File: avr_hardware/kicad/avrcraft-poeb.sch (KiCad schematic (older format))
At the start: 61 parts, among them J1 AVRISP6, J2 AVRISP6, P1 ETHERNET, P4 GND, P5 PD34, P6 5V, P7 3V3, P8 PB0, Q1 SQ2361EES-T1-GE3CT-ND, T1 S553-5999-52, U1 ATMEGA328, U2 MCP1824v3.3, U3 ENC424J600, U4 A4447SLJTR, X1 XTAL4P, X2 25MHz

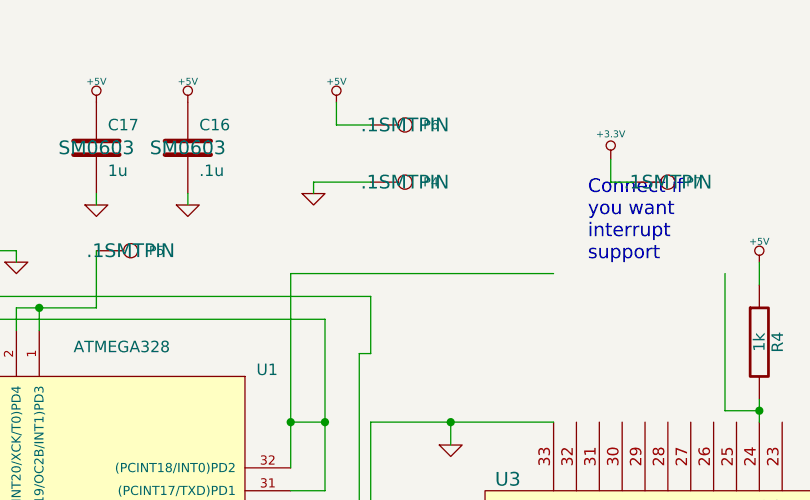
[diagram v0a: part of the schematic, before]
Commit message: update poc
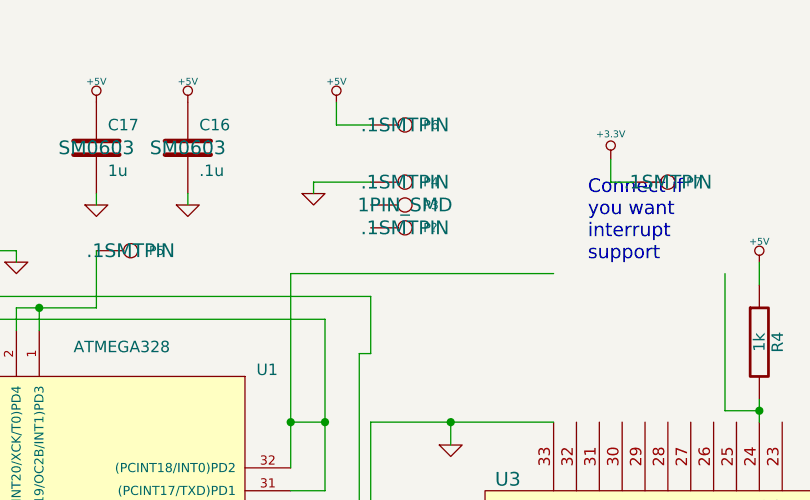
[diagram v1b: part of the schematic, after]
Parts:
- added P3: GND, 1PIN_SMD, symbol CONN_1
- added P?: GND, .1SMTPIN, symbol CONN_1
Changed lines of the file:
@@
-EESchema Schematic File Version 2  date Wed 27 Nov 2013 03:16:10 PM EST
+EESchema Schematic File Version 2  date Tue 04 Feb 2014 05:22:17 PM EST
 LIBS:power
 LIBS:device
@@
 Sheet 1 1
 Title ""
-Date "27 nov 2013"
+Date "4 feb 2014"
 Rev ""
 Comp ""
@@
 Connection ~ 1850 550
 $Comp
-L GND #PWR01
+L CONN_1 P?
+U 1 1 52F167B0
+P 5400 1450
+F 0 "P?" H 5480 1450 40  0000 L CNN
+F 1 "GND" H 5400 1505 30  0001 C CNN
+F 2 ".1SMTPIN" H 5400 1450 60  0000 C CNN
+	1    5400 1450
+	1    0    0    -1
+$EndComp
+$Comp
+L CONN_1 P3
+U 1 1 52F167AD
+P 5400 1350
+F 0 "P3" H 5480 1350 40  0000 L CNN
+F 1 "GND" H 5400 1405 30  0001 C CNN
+F 2 "1PIN_SMD" H 5400 1350 60  0000 C CNN
+	1    5400 1350
+	1    0    0    -1
+$EndComp
+$Comp
+L GND #PWR4
 U 1 1 52054D0F
 P 1950 1650
-F 0 "#PWR01" H 1950 1650 30  0001 C CNN
+F 0 "#PWR4" H 1950 1650 30  0001 C CNN
 F 1 "GND" H 1950 1580 30  0001 C CNN
 	1    1950 1650
@@
 $EndComp
 $Comp
-L +3.3V #PWR02
+L +3.3V #PWR3
 U 1 1 51D472BC
 P 1750 1900
-F 0 "#PWR02" H 1750 1860 30  0001 C CNN
+F 0 "#PWR3" H 1750 1860 30  0001 C CNN
 F 1 "+3.3V" H 1750 2010 30  0000 C CNN
 	1    1750 1900
@@
 $EndComp
 $Comp
-L GND #PWR03
+L GND #PWR31
 U 1 1 510EC704
 P 8000 2650
-F 0 "#PWR03" H 8000 2650 30  0001 C CNN
+F 0 "#PWR31" H 8000 2650 30  0001 C CNN
 F 1 "GND" H 8000 2580 30  0001 C CNN
 	1    8000 2650
@@
 Connect if \nyou want\ninterrupt\nsupport
 $Comp
-L +5V #PWR04
+L +5V #PWR24
 U 1 1 510EAED6
 P 6950 1600
-F 0 "#PWR04" H 6950 1690 20  0001 C CNN
+F 0 "#PWR24" H 6950 1690 20  0001 C CNN
 F 1 "+5V" H 6950 1690 30  0000 C CNN
 	1    6950 1600
@@
 $EndComp
 $Comp
-L +5V #PWR05
+L +5V #PWR11
 U 1 1 5109F491
 P 4050 900
-F 0 "#PWR05" H 4050 990 20  0001 C CNN
+F 0 "#PWR11" H 4050 990 20  0001 C CNN
 F 1 "+5V" H 4050 990 30  0000 C CNN
 	1    4050 900
@@
 $EndComp
 $Comp
-L GND #PWR06
+L GND #PWR12
 U 1 1 5109F490
 P 4050 1350
-F 0 "#PWR06" H 4050 1350 30  0001 C CNN
+F 0 "#PWR12" H 4050 1350 30  0001 C CNN
 F 1 "GND" H 4050 1280 30  0001 C CNN
 	1    4050 1350
@@
 NOTE: 5v Rail should be roughly 4.5V
 $Comp
-L GND #PWR07
+L GND #PWR14
 U 1 1 51031CF0
 P 4450 1350
-F 0 "#PWR07" H 4450 1350 30  0001 C CNN
+F 0 "#PWR14" H 4450 1350 30  0001 C CNN
 F 1 "GND" H 4450 1280 30  0001 C CNN
 	1    4450 1350
@@
 $EndComp
 $Comp
-L +5V #PWR08
+L +5V #PWR13
 U 1 1 51031CE7
 P 4450 900
-F 0 "#PWR08" H 4450 990 20  0001 C CNN
+F 0 "#PWR13" H 4450 990 20  0001 C CNN
 F 1 "+5V" H 4450 990 30  0000 C CNN
 	1    4450 900
@@
 $EndComp
 $Comp
-L +5V #PWR09
+L +5V #PWR16
 U 1 1 5102E4BB
 P 5100 900
-F 0 "#PWR09" H 5100 990 20  0001 C CNN
+F 0 "#PWR16" H 5100 990 20  0001 C CNN
 F 1 "+5V" H 5100 990 30  0000 C CNN
 	1    5100 900
@@
 $EndComp
 $Comp
-L +3.3V #PWR010
+L +3.3V #PWR22
 U 1 1 5102E4A4
 P 6300 1150
-F 0 "#PWR010" H 6300 1110 30  0001 C CNN
+F 0 "#PWR22" H 6300 1110 30  0001 C CNN
 F 1 "+3.3V" H 6300 1260 30  0000 C CNN
 	1    6300 1150
@@
 $EndComp
 $Comp
-L GND #PWR011
+L GND #PWR15
 U 1 1 5102E175
 P 5000 1300
-F 0 "#PWR011" H 5000 1300 30  0001 C CNN
+F 0 "#PWR15" H 5000 1300 30  0001 C CNN
 F 1 "GND" H 5000 1230 30  0001 C CNN
 	1    5000 1300
@@
 HighCOut
 $Comp
-L +5V #PWR012
+L +5V #PWR32
 U 1 1 5101B419
 P 8150 6850
-F 0 "#PWR012" H 8150 6940 20  0001 C CNN
+F 0 "#PWR32" H 8150 6940 20  0001 C CNN
 F 1 "+5V" H 8150 6940 30  0000 C CNN
 	1    8150 6850
@@
 $EndComp
 $Comp
-L GND #PWR013
+L GND #PWR21
 U 1 1 5101B3F2
 P 5700 7250
-F 0 "#PWR013" H 5700 7250 30  0001 C CNN
+F 0 "#PWR21" H 5700 7250 30  0001 C CNN
 F 1 "GND" H 5700 7180 30  0001 C CNN
 	1    5700 7250
@@
 POE+
 $Comp
-L GND #PWR014
+L GND #PWR34
 U 1 1 510061F7
 P 8750 6150
-F 0 "#PWR014" H 8750 6150 30  0001 C CNN
+F 0 "#PWR34" H 8750 6150 30  0001 C CNN
 F 1 "GND" H 8750 6080 30  0001 C CNN
 	1    8750 6150
@@
 $EndComp
 $Comp
-L GND #PWR015
+L GND #PWR35
 U 1 1 51005EDF
 P 10450 3050
-F 0 "#PWR015" H 10450 3050 30  0001 C CNN
+F 0 "#PWR35" H 10450 3050 30  0001 C CNN
 F 1 "GND" H 10450 2980 30  0001 C CNN
 	1    10450 3050
@@
 $EndComp
 $Comp
-L +3.3V #PWR016
+L +3.3V #PWR29
 U 1 1 50FE1DE9
 P 7950 5250
-F 0 "#PWR016" H 7950 5210 30  0001 C CNN
+F 0 "#PWR29" H 7950 5210 30  0001 C CNN
 F 1 "+3.3V" H 7950 5360 30  0000 C CNN
 	1    7950 5250
@@
 $EndComp
 $Comp
-L GND #PWR017
+L GND #PWR30
 U 1 1 50FE1DDF
 P 7950 5700
-F 0 "#PWR017" H 7950 5700 30  0001 C CNN
+F 0 "#PWR30" H 7950 5700 30  0001 C CNN
 F 1 "GND" H 7950 5630 30  0001 C CNN
 	1    7950 5700
@@
 $EndComp
 $Comp
-L GND #PWR018
+L GND #PWR33
 U 1 1 50FE1DDB
 P 8650 5000
-F 0 "#PWR018" H 8650 5000 30  0001 C CNN
+F 0 "#PWR33" H 8650 5000 30  0001 C CNN
 F 1 "GND" H 8650 4930 30  0001 C CNN
 	1    8650 5000
@@
 $EndComp
 $Comp
-L +3.3V #PWR019
+L +3.3V #PWR27
 U 1 1 50FDE179
 P 7750 2700
-F 0 "#PWR019" H 7750 2660 30  0001 C CNN
+F 0 "#PWR27" H 7750 2660 30  0001 C CNN
 F 1 "+3.3V" H 7750 2810 30  0000 C CNN
 	1    7750 2700
@@
 $EndComp
 $Comp
-L GND #PWR020
+L GND #PWR28
 U 1 1 50FDE152
 P 7800 4050
-F 0 "#PWR020" H 7800 4050 30  0001 C CNN
+F 0 "#PWR28" H 7800 4050 30  0001 C CNN
 F 1 "GND" H 7800 3980 30  0001 C CNN
 	1    7800 4050
@@
 $EndComp
 $Comp
-L GND #PWR021
+L GND #PWR26
 U 1 1 50FDE072
 P 7400 5150
-F 0 "#PWR021" H 7400 5150 30  0001 C CNN
+F 0 "#PWR26" H 7400 5150 30  0001 C CNN
 F 1 "GND" H 7400 5080 30  0001 C CNN
 	1    7400 5150
@@
 $EndComp
 $Comp
-L +5V #PWR022
+L +5V #PWR9
 U 1 1 50FDE020
 P 3700 4950
-F 0 "#PWR022" H 3700 5040 20  0001 C CNN
+F 0 "#PWR9" H 3700 5040 20  0001 C CNN
 F 1 "+5V" H 3700 5040 30  0000 C CNN
 	1    3700 4950
@@
 $EndComp
 $Comp
-L GND #PWR023
+L GND #PWR10
 U 1 1 50FDE01D
 P 3700 5050
-F 0 "#PWR023" H 3700 5050 30  0001 C CNN
+F 0 "#PWR10" H 3700 5050 30  0001 C CNN
 F 1 "GND" H 3700 4980 30  0001 C CNN
 	1    3700 5050
@@
 $EndComp
 $Comp
-L +3.3V #PWR024
+L +3.3V #PWR19
 U 1 1 50FDE008
 P 5600 4050
-F 0 "#PWR024" H 5600 4010 30  0001 C CNN
+F 0 "#PWR19" H 5600 4010 30  0001 C CNN
 F 1 "+3.3V" H 5600 4160 30  0000 C CNN
 	1    5600 4050
@@
 $EndComp
 $Comp
-L +3.3V #PWR025
+L +3.3V #PWR17
 U 1 1 50FDE003
 P 5300 4850
-F 0 "#PWR025" H 5300 4810 30  0001 C CNN
+F 0 "#PWR17" H 5300 4810 30  0001 C CNN
 F 1 "+3.3V" H 5300 4960 30  0000 C CNN
 	1    5300 4850
@@
 $EndComp
 $Comp
-L +3.3V #PWR026
+L +3.3V #PWR23
 U 1 1 50FDDFFD
 P 6700 4650
-F 0 "#PWR026" H 6700 4610 30  0001 C CNN
+F 0 "#PWR23" H 6700 4610 30  0001 C CNN
 F 1 "+3.3V" H 6700 4760 30  0000 C CNN
 	1    6700 4650
@@
 $EndComp
 $Comp
-L GND #PWR027
+L GND #PWR25
 U 1 1 50FDDFE7
 P 6950 5600
-F 0 "#PWR027" H 6950 5600 30  0001 C CNN
+F 0 "#PWR25" H 6950 5600 30  0001 C CNN
 F 1 "GND" H 6950 5530 30  0001 C CNN
 	1    6950 5600
@@
 $EndComp
 $Comp
-L GND #PWR028
+L GND #PWR20
 U 1 1 50FDDF6F
 P 5650 5450
-F 0 "#PWR028" H 5650 5450 30  0001 C CNN
+F 0 "#PWR20" H 5650 5450 30  0001 C CNN
 F 1 "GND" H 5650 5380 30  0001 C CNN
 	1    5650 5450
@@
 $EndComp
 $Comp
-L GND #PWR029
+L GND #PWR18
 U 1 1 50FDDEFB
 P 5600 2400
-F 0 "#PWR029" H 5600 2400 30  0001 C CNN
+F 0 "#PWR18" H 5600 2400 30  0001 C CNN
 F 1 "GND" H 5600 2330 30  0001 C CNN
 	1    5600 2400
@@
 $EndComp
 $Comp
-L GND #PWR030
+L GND #PWR8
 U 1 1 50FDDD8F
 P 3700 1600
-F 0 "#PWR030" H 3700 1600 30  0001 C CNN
+F 0 "#PWR8" H 3700 1600 30  0001 C CNN
 F 1 "GND" H 3700 1530 30  0001 C CNN
 	1    3700 1600
@@
 $EndComp
 $Comp
-L +5V #PWR031
+L +5V #PWR6
 U 1 1 50FDDD86
 P 3500 1650
-F 0 "#PWR031" H 3500 1740 20  0001 C CNN
+F 0 "#PWR6" H 3500 1740 20  0001 C CNN
 F 1 "+5V" H 3500 1740 30  0000 C CNN
 	1    3500 1650
@@
 $EndComp
 $Comp
-L +5V #PWR032
+L +5V #PWR5
 U 1 1 50FDDD79
 P 3100 4050
-F 0 "#PWR032" H 3100 4140 20  0001 C CNN
+F 0 "#PWR5" H 3100 4140 20  0001 C CNN
 F 1 "+5V" H 3100 4140 30  0000 C CNN
 	1    3100 4050
@@
 $EndComp
 $Comp
-L GND #PWR033
+L GND #PWR7
 U 1 1 50FDDD69
 P 3600 4050
-F 0 "#PWR033" H 3600 4050 30  0001 C CNN
+F 0 "#PWR7" H 3600 4050 30  0001 C CNN
 F 1 "GND" H 3600 3980 30  0001 C CNN
 	1    3600 4050
@@
 $EndComp
 $Comp
-L +5V #PWR034
+L +5V #PWR1
 U 1 1 50FDDB58
 P 1050 2950
-F 0 "#PWR034" H 1050 3040 20  0001 C CNN
+F 0 "#PWR1" H 1050 3040 20  0001 C CNN
 F 1 "+5V" H 1050 3040 30  0000 C CNN
 	1    1050 2950
@@
 $EndComp
 $Comp
-L GND #PWR035
+L GND #PWR2
 U 1 1 50FDDB44
 P 1400 3100
-F 0 "#PWR035" H 1400 3100 30  0001 C CNN
+F 0 "#PWR2" H 1400 3100 30  0001 C CNN
 F 1 "GND" H 1400 3030 30  0001 C CNN
 	1    1400 3100
